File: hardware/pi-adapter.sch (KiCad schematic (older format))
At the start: 32 parts, among them P1 CONN_01X04, P10 CONN_01X04, P11 CONN_01X04, P12 CONN_01X04, P13 CONN_01X04, P14 CONN_01X04, P15 CONN_01X04, P16 CONN_01X04, P2 +5V, P2 CONN_01X04, P20 CONN_02X20, P21 CONN_01X03, P22 CONN_01X06, P23 CONN_01X03, P3 CONN_01X04, P4 CONN_01X04, P4 GND, P5 CONN_01X04, P6 CONN_01X04, P7 CONN_01X04, P8 CONN_01X04, P9 CONN_01X04, U1 74HCT245, U2 74HCT245, U3 74HCT245, U4 74HCT245

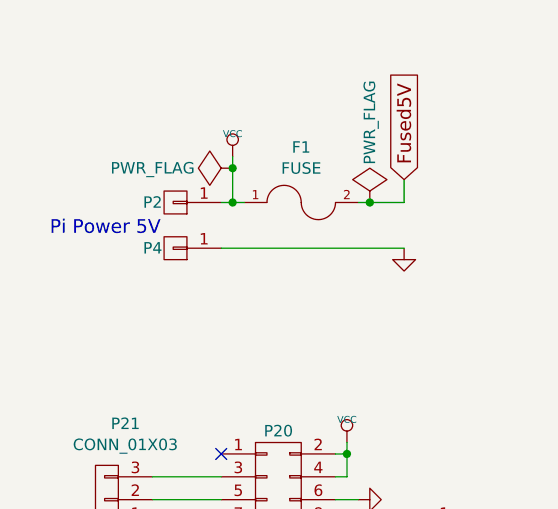
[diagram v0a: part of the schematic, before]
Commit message: o Some more renaming needed.
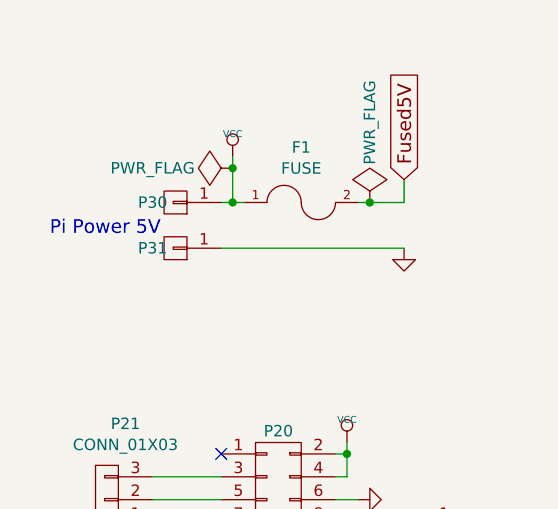
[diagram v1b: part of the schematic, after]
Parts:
- renumbered P2 to P30, P4 to P31
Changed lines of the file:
@@
 NoConn ~ 1900 3500
 $Comp
-L PWR_FLAG #FLG017
+L PWR_FLAG #FLG016
 U 1 1 557B23A7
 P 1850 4700
-F 0 "#FLG017" H 1850 4795 50  0001 C CNN
+F 0 "#FLG016" H 1850 4795 50  0001 C CNN
 F 1 "PWR_FLAG" H 1850 4880 50  0000 C CNN
 F 2 "" H 1850 4700 60  0000 C CNN
@@
 Connection ~ 1850 4600
 $Comp
-L GND #PWR018
+L GND #PWR017
 U 1 1 562B120F
 P 2700 1800
-F 0 "#PWR018" H 2700 1800 30  0001 C CNN
+F 0 "#PWR017" H 2700 1800 30  0001 C CNN
 F 1 "GND" H 2700 1730 30  0001 C CNN
 F 2 "" H 2700 1800 60  0000 C CNN
@@
 $EndComp
 $Comp
-L VCC #PWR019
+L VCC #PWR018
 U 1 1 562B12CC
 P 1950 1400
-F 0 "#PWR019" H 1950 1500 30  0001 C CNN
+F 0 "#PWR018" H 1950 1500 30  0001 C CNN
 F 1 "VCC" H 1950 1500 30  0000 C CNN
 F 2 "" H 1950 1400 60  0000 C CNN
@@
 $EndComp
 $Comp
-L CONN_01X01 P2
+L CONN_01X01 P30
 U 1 1 562B3873
 P 1700 1600
-F 0 "P2" H 1800 1600 50  0000 C CNN
+F 0 "P30" H 1800 1600 50  0000 C CNN
 F 1 "+5V" V 1800 1600 50  0001 C CNN
 F 2 "Pin_Headers:Pin_Header_Straight_1x01" H 1700 1600 60  0001 C CNN
@@
 $EndComp
 $Comp
-L CONN_01X01 P4
+L CONN_01X01 P31
 U 1 1 562B38C3
 P 1700 1800
-F 0 "P4" H 1800 1800 50  0000 C CNN
+F 0 "P31" H 1800 1800 50  0000 C CNN
 F 1 "GND" V 1800 1800 50  0001 C CNN
 F 2 "Pin_Headers:Pin_Header_Straight_1x01" H 1700 1800 60  0001 C CNN
@@
 	5900 1350 5900 1850
 $Comp
-L GND #PWR020
+L GND #PWR019
 U 1 1 56C176D3
 P 6400 1750
-F 0 "#PWR020" H 6400 1750 30  0001 C CNN
+F 0 "#PWR019" H 6400 1750 30  0001 C CNN
 F 1 "GND" H 6400 1680 30  0001 C CNN
 F 2 "" H 6400 1750 60  0000 C CNN
@@
 $EndComp
 $Comp
-L GND #PWR021
+L GND #PWR020
 U 1 1 56C198BA
 P 2800 3300
-F 0 "#PWR021" H 2800 3300 30  0001 C CNN
+F 0 "#PWR020" H 2800 3300 30  0001 C CNN
 F 1 "GND" H 2800 3230 30  0001 C CNN
 F 2 "" H 2800 3300 60  0000 C CNN
@@
 	1600 2900 1900 2900
 $Comp
-L GND #PWR022
+L GND #PWR021
 U 1 1 56C19EE1
 P 1600 3100
-F 0 "#PWR022" H 1600 3100 30  0001 C CNN
+F 0 "#PWR021" H 1600 3100 30  0001 C CNN
 F 1 "GND" H 1600 3030 30  0001 C CNN
 F 2 "" H 1600 3100 60  0000 C CNN
@@
 Connection ~ 1950 1600
 $Comp
-L VCC #PWR023
+L VCC #PWR022
 U 1 1 56C22E4F
 P 2450 2650
-F 0 "#PWR023" H 2450 2750 30  0001 C CNN
+F 0 "#PWR022" H 2450 2750 30  0001 C CNN
 F 1 "VCC" H 2450 2750 30  0000 C CNN
 F 2 "" H 2450 2650 60  0000 C CNN
@@
 	5900 3050 5900 3550
 $Comp
-L GND #PWR024
+L GND #PWR023
 U 1 1 56C22C65
 P 6400 3450
-F 0 "#PWR024" H 6400 3450 30  0001 C CNN
+F 0 "#PWR023" H 6400 3450 30  0001 C CNN
 F 1 "GND" H 6400 3380 30  0001 C CNN
 F 2 "" H 6400 3450 60  0000 C CNN
@@
 	5900 4750 5900 5250
 $Comp
-L GND #PWR025
+L GND #PWR024
 U 1 1 56C22D48
 P 6400 5150
-F 0 "#PWR025" H 6400 5150 30  0001 C CNN
+F 0 "#PWR024" H 6400 5150 30  0001 C CNN
 F 1 "GND" H 6400 5080 30  0001 C CNN
 F 2 "" H 6400 5150 60  0000 C CNN
@@
 	5900 6550 5900 7050
 $Comp
-L GND #PWR026
+L GND #PWR025
 U 1 1 56C22F13
 P 6400 6950
-F 0 "#PWR026" H 6400 6950 30  0001 C CNN
+F 0 "#PWR025" H 6400 6950 30  0001 C CNN
 F 1 "GND" H 6400 6880 30  0001 C CNN
 F 2 "" H 6400 6950 60  0000 C CNN
@@
 SCLK
 $Comp
-L PWR_FLAG #FLG?
+L PWR_FLAG #FLG026
 U 1 1 56CA81D8
 P 2550 1600
-F 0 "#FLG?" H 2550 1695 50  0001 C CNN
+F 0 "#FLG026" H 2550 1695 50  0001 C CNN
 F 1 "PWR_FLAG" V 2550 1950 50  0000 C CNN
 F 2 "" H 2550 1600 60  0000 C CNN
@@
 	1950 1400 1950 1600
 $Comp
-L PWR_FLAG #FLG?
+L PWR_FLAG #FLG027
 U 1 1 56CA8545
 P 1950 1450
-F 0 "#FLG?" H 1950 1545 50  0001 C CNN
+F 0 "#FLG027" H 1950 1545 50  0001 C CNN
 F 1 "PWR_FLAG" V 1950 1800 50  0000 C CNN
 F 2 "" H 1950 1450 60  0000 C CNN
@@
 	2400 2700 2450 2700
 $Comp
-L GND #PWR?
+L GND #PWR028
 U 1 1 56CF0349
 P 2500 4100
-F 0 "#PWR?" H 2500 4100 30  0001 C CNN
+F 0 "#PWR028" H 2500 4100 30  0001 C CNN
 F 1 "GND" H 2500 4030 30  0001 C CNN
 F 2 "" H 2500 4100 60  0000 C CNN
